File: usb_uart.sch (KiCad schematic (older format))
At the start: 13 parts, among them P2 CONN_01X06, U20 CP2102N-A01-GQFN28, U25 CM1293A-04SO

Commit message: Almost all components has placed.
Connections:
- wire segments 80 -> 78
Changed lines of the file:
@@
 EESchema Schematic File Version 4
 LIBS:dotmatrix_64x48-cache
-EELAYER 28 0
+EELAYER 29 0
 EELAYER END
 $Descr A4 11693 8268
@@
 Wire Wire Line
 	3800 1300 3800 1250
-Connection ~ 3800 1250
 Wire Wire Line
 	4000 1300 4000 1250
@@
 	4200 1250 4400 1250
 $Comp
-L power:GND #PWR022
-U 1 1 5BBD8B5F
-P 3500 1400
-F 0 "#PWR022" H 3500 1150 50  0001 C CNN
-F 1 "GND" H 3505 1227 50  0000 C CNN
-F 2 "" H 3500 1400 50  0001 C CNN
-F 3 "" H 3500 1400 50  0001 C CNN
-	1    3500 1400
-	1    0    0    -1
-$EndComp
-Wire Wire Line
-	3500 1400 3500 1250
-Wire Wire Line
-	3500 1250 3800 1250
-$Comp
 L power:GND #PWR052

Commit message: Too less PCB space.
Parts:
- P2: footprint Pin_Headers:Pin_Header_Straight_1x08_Pitch2.54mm -> Pin_Headers:Pin_Header_Straight_1x06_Pitch2.54mm
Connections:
- net labels added: DTR, E_RX, E_TX, RTS, VBUS
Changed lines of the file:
@@
 F 0 "P2" H 7127 1936 50  0000 L CNN
 F 1 "CONN_01X06" H 7127 1845 50  0000 L CNN
-F 2 "Pin_Headers:Pin_Header_Straight_1x08_Pitch2.54mm" H 7127 1754 50  0000 L CNN
+F 2 "Pin_Headers:Pin_Header_Straight_1x06_Pitch2.54mm" H 7127 1754 50  0000 L CNN
 F 3 "" H 7050 1850 50  0000 C CNN
 	1    7050 1850
@@
 	3450 3750 3450 3550
 Connection ~ 3450 3750
+Text GLabel 6850 1950 0    60   Input ~ 0
+E_TX
+Text GLabel 6850 1850 0    60   Input ~ 0
+E_RX
+Text GLabel 6850 2150 0    60   Input ~ 0
+RTS
+Text GLabel 6850 2050 0    60   Input ~ 0
+DTR
+Text Label 2550 2500 0    50   ~ 0
+VBUS
 $EndSCHEMATC

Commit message: Switched to new kicad libraries
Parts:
- C67, C69, C70, C71, C73, C74: symbol device:C -> dotmatrix_64x48-rescue:C-device
- CONN2: symbol Connector:USB_OTG -> dotmatrix_64x48-rescue:USB_OTG-Connector
- D13: symbol device:LED_Small -> dotmatrix_64x48-rescue:LED_Small-device
- P2: symbol Connector:Conn_01x06 -> dotmatrix_64x48-rescue:Conn_01x06-Connector
- R116, R117: symbol device:R -> dotmatrix_64x48-rescue:R-device
- U25: symbol ESD_Protection:SRV05-4 -> dotmatrix_64x48-rescue:SRV05-4-ESD_Protection
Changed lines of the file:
@@
 $EndComp
 $Comp
-L device:C C71
+L dotmatrix_64x48-rescue:C-device C71
 U 1 1 5BBCC45B
 P 4000 2350
@@
 $EndComp
 $Comp
-L device:C C69
+L dotmatrix_64x48-rescue:C-device C69
 U 1 1 5BBCC461
 P 3800 2350
@@
 $EndComp
 $Comp
-L device:C C74
+L dotmatrix_64x48-rescue:C-device C74
 U 1 1 5BBCC467
 P 4200 2350
@@
 	4450 2150 4200 2150
 $Comp
-L device:C C70
+L dotmatrix_64x48-rescue:C-device C70
 U 1 1 5BBD1F28
 P 4000 1450
@@
 $EndComp
 $Comp
-L device:C C67
+L dotmatrix_64x48-rescue:C-device C67
 U 1 1 5BBD1F2E
 P 3800 1450
@@
 $EndComp
 $Comp
-L device:C C73
+L dotmatrix_64x48-rescue:C-device C73
 U 1 1 5BBD1F34
 P 4200 1450
@@
 	4200 1250 4400 1250
 $Comp
-L power:GND #PWR052
+L dotmatrix_64x48-rescue:GND-power #PWR052
 U 1 1 5BBDC36A
 P 4200 1600
@@
 $EndComp
 $Comp
-L power:GND #PWR026
+L dotmatrix_64x48-rescue:GND-power #PWR026
 U 1 1 5BBDF9D0
 P 4000 1600
@@
 $EndComp
 $Comp
-L power:GND #PWR023
+L dotmatrix_64x48-rescue:GND-power #PWR023
 U 1 1 5BBE3036
 P 3800 1600
@@
 $EndComp
 $Comp
-L power:GND #PWR053
+L dotmatrix_64x48-rescue:GND-power #PWR053
 U 1 1 5BBE9D25
 P 4200 2500
@@
 $EndComp
 $Comp
-L power:GND #PWR051
+L dotmatrix_64x48-rescue:GND-power #PWR051
 U 1 1 5BBE9D2B
 P 4000 2500
@@
 $EndComp
 $Comp
-L power:GND #PWR025
+L dotmatrix_64x48-rescue:GND-power #PWR025
 U 1 1 5BBE9D31
 P 3800 2500
@@
 $EndComp
 $Comp
-L Connector:USB_OTG CONN?
+L dotmatrix_64x48-rescue:USB_OTG-Connector CONN?
 U 1 1 5BBED423
 P 2100 2700
@@
 	2000 3200 2050 3200
 $Comp
-L power:GND #PWR019
+L dotmatrix_64x48-rescue:GND-power #PWR019
 U 1 1 5BBF16CE
 P 2050 3200
@@
 USBDN
 $Comp
-L power:GND #PWR054
+L dotmatrix_64x48-rescue:GND-power #PWR054
 U 1 1 5BC0208A
 P 5350 3600
@@
 $EndComp
 $Comp
-L power:GND #PWR067
+L dotmatrix_64x48-rescue:GND-power #PWR067
 U 1 1 5BC069E8
 P 5450 3600
@@
 $EndComp
 $Comp
-L device:R R117
+L dotmatrix_64x48-rescue:R-device R117
 U 1 1 5BC0FE7D
 P 4550 1550
@@
 	4400 1250 5350 1250
 $Comp
-L device:LED_Small D13
+L dotmatrix_64x48-rescue:LED_Small-device D13
 U 1 1 5BC197DC
 P 2850 1850
@@
 $EndComp
 $Comp
-L device:R R116
+L dotmatrix_64x48-rescue:R-device R116
 U 1 1 5BC197E2
 P 3250 1850
@@
 	3100 1850 2950 1850
 $Comp
-L power:GND #PWR020
+L dotmatrix_64x48-rescue:GND-power #PWR020
 U 1 1 5BC2860D
 P 2550 1850
@@
 	4600 1950 4850 1950
 $Comp
-L Connector:Conn_01x06 P2
+L dotmatrix_64x48-rescue:Conn_01x06-Connector P2
 U 1 1 5BC37DD7
 P 7050 1850
@@
 USB3V3
 $Comp
-L power:GND #PWR068
+L dotmatrix_64x48-rescue:GND-power #PWR068
 U 1 1 5BC42F9C
 P 6400 1750
@@
 NoConn ~ 4850 1850
 $Comp
-L ESD_Protection:SRV05-4 U25
+L dotmatrix_64x48-rescue:SRV05-4-ESD_Protection U25
 U 1 1 5C65572B
 P 2950 3650
@@
 $EndComp
 $Comp
-L power:GND #PWR0136
+L dotmatrix_64x48-rescue:GND-power #PWR0136
 U 1 1 5C655732
 P 2950 4150

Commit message: Before removing old style stitching vias
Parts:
- removed P2: CONN_01X06, Pin_Headers:Pin_Header_Straight_1x06_Pitch2.54mm, symbol dotmatrix_64x48-rescue:Conn_01x06-Connector
- C67, C69: value 10u -> 10u 10V; footprint Capacitors_SMD:C_0603_HandSoldering -> Capacitor_SMD:C_0603_1608Metric_Pad1.05x0.95mm_HandSolder
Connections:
- wire segments 78 -> 75
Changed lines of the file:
@@
 P 3800 2350
 F 0 "C69" H 3750 1950 50  0000 L CNN
-F 1 "10u" H 3750 1850 50  0000 L CNN
-F 2 "Capacitors_SMD:C_0603_HandSoldering" H 3915 2259 50  0001 L CNN
+F 1 "10u 10V" V 3650 1850 50  0000 L CNN
+F 2 "Capacitor_SMD:C_0603_1608Metric_Pad1.05x0.95mm_HandSolder" H 3915 2259 50  0001 L CNN
 F 3 "" H 3800 2350 50  0000 C CNN
 	1    3800 2350
@@
 P 3800 1450
 F 0 "C67" H 3750 1050 50  0000 L CNN
-F 1 "10u" H 3750 950 50  0000 L CNN
-F 2 "Capacitors_SMD:C_0603_HandSoldering" H 3915 1359 50  0001 L CNN
+F 1 "10u 10V" V 3650 950 50  0000 L CNN
+F 2 "Capacitor_SMD:C_0603_1608Metric_Pad1.05x0.95mm_HandSolder" H 3915 1359 50  0001 L CNN
 F 3 "" H 3800 1450 50  0000 C CNN
 	1    3800 1450
@@
 Wire Wire Line
 	4600 1950 4850 1950
-$Comp
-L dotmatrix_64x48-rescue:Conn_01x06-Connector P2
-U 1 1 5BC37DD7
-P 7050 1850
-F 0 "P2" H 7127 1936 50  0000 L CNN
-F 1 "CONN_01X06" H 7127 1845 50  0000 L CNN
-F 2 "Pin_Headers:Pin_Header_Straight_1x06_Pitch2.54mm" H 7127 1754 50  0000 L CNN
-F 3 "" H 7050 1850 50  0000 C CNN
-	1    7050 1850
-	1    0    0    -1
-$EndComp
-Wire Wire Line
-	6850 1650 6600 1650
-Wire Wire Line
-	6600 1650 6600 1250
 Wire Wire Line
 	6600 1250 5350 1250
 Connection ~ 5350 1250
-Text Label 6150 1250 0    50   ~ 0
+Text Label 6600 1250 0    50   ~ 0
 USB3V3
-$Comp
-L dotmatrix_64x48-rescue:GND-power #PWR068
-U 1 1 5BC42F9C
-P 6400 1750
-F 0 "#PWR068" H 6400 1500 50  0001 C CNN
-F 1 "GND" H 6405 1577 50  0000 C CNN
-F 2 "" H 6400 1750 50  0001 C CNN
-F 3 "" H 6400 1750 50  0001 C CNN
-	1    6400 1750
-	1    0    0    -1
-$EndComp
-Wire Wire Line
-	6400 1750 6850 1750
 Wire Wire Line
 	6850 1850 6550 1850
@@
 	3450 3750 3450 3550
 Connection ~ 3450 3750
-Text GLabel 6850 1950 0    60   Input ~ 0
+Text GLabel 6850 1950 2    60   Input ~ 0
 E_TX
-Text GLabel 6850 1850 0    60   Input ~ 0
+Text GLabel 6850 1850 2    60   Input ~ 0
 E_RX
-Text GLabel 6850 2150 0    60   Input ~ 0
+Text GLabel 6850 2150 2    60   Input ~ 0
 RTS
-Text GLabel 6850 2050 0    60   Input ~ 0
+Text GLabel 6850 2050 2    60   Input ~ 0
 DTR
 Text Label 2550 2500 0    50   ~ 0

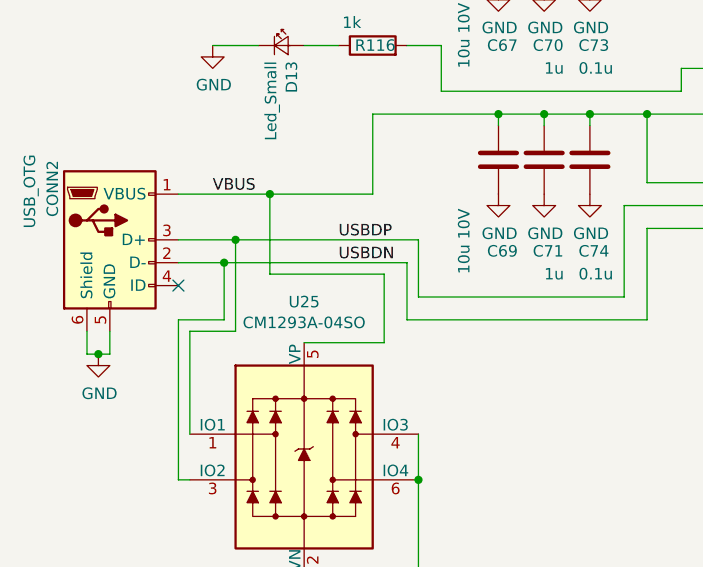
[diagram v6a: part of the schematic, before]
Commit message: Design update
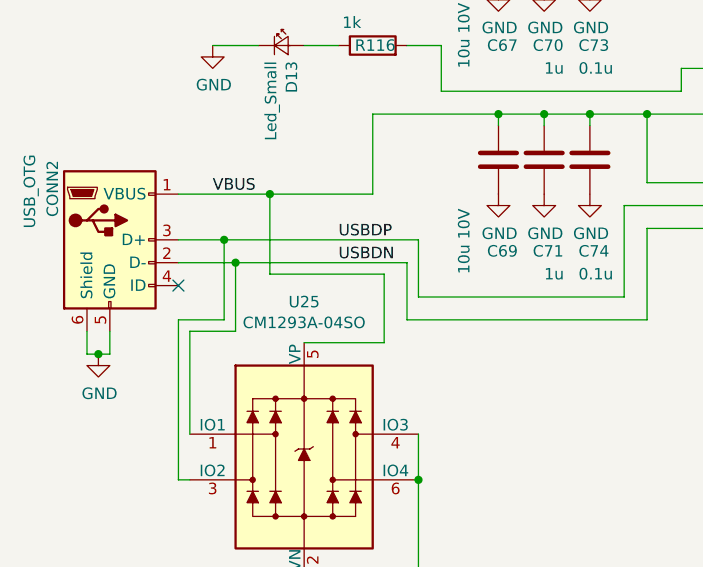
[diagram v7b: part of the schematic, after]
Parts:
- CONN2: footprint components:USB-MICRO-B-RECEPT-UNIVERSAL -> components:USB_Micro-B_Jing_A01SB141B1-067
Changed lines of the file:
@@
 F 0 "CONN2" V 1850 2800 50  0000 L CNN
 F 1 "USB_OTG" V 1750 2750 50  0000 L CNN
-F 2 "components:USB-MICRO-B-RECEPT-UNIVERSAL" V 2086 2888 50  0001 L CNN
+F 2 "components:USB_Micro-B_Jing_A01SB141B1-067" V 2086 2888 50  0001 L CNN
 F 3 "" V 2050 2600 50  0000 C CNN
 	1    2100 2700
@@
 	6150 1750 6050 1750
 Wire Wire Line
-	2400 2800 2600 2800
-Connection ~ 2600 2800
-Wire Wire Line
 	2800 2850 2800 2500
 Wire Wire Line
@@
 	2800 2500 2400 2500
 Connection ~ 2800 2500
-Wire Wire Line
-	2600 2800 3400 2800
 NoConn ~ 6050 1550
 NoConn ~ 6050 1650
@@
 	2400 3750 2450 3750
 Wire Wire Line
-	2600 2800 2600 3050
-Wire Wire Line
-	2400 2700 2650 2700
-Wire Wire Line
 	2450 3100 2650 3100
-Wire Wire Line
-	2650 3100 2650 2700
-Connection ~ 2650 2700
-Wire Wire Line
-	2650 2700 3450 2700
 Wire Wire Line
 	3300 2850 3300 3150
@@
 Text Label 2550 2500 0    50   ~ 0
 VBUS
+Wire Wire Line
+	2400 2700 2600 2700
+Wire Wire Line
+	2400 2800 2650 2800
+Wire Wire Line
+	2600 3050 2600 2700
+Connection ~ 2600 2700
+Wire Wire Line
+	2600 2700 3450 2700
+Wire Wire Line
+	2650 3100 2650 2800
+Connection ~ 2650 2800
+Wire Wire Line
+	2650 2800 3400 2800
 $EndSCHEMATC

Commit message: Almost done drawing pcb tracks
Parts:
- R116: value 1k -> 4.7k
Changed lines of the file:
@@
 P 3250 1850
 F 0 "R116" V 3250 1750 50  0000 L CNN
-F 1 "1k" V 3350 1900 50  0000 L CNN
+F 1 "4.7k" V 3350 1900 50  0000 L CNN
 F 2 "Resistors_SMD:R_0603_HandSoldering" V 3180 1850 50  0001 C CNN
 F 3 "" H 3250 1850 50  0000 C CNN
